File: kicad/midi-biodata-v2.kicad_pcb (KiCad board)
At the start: 2 copper layers, 63.5 x 45.7 mm, 37 parts, among them J1 DIN-5_180degree, J2 Audio-Jack-2, J3 Conn_01x02, J4 Conn_01x02, SW1 SW_Push, U1 ATMEGA328P-AU, U2 POT_SWITCH, U3 LMC555xM, Y1 Crystal_GND2

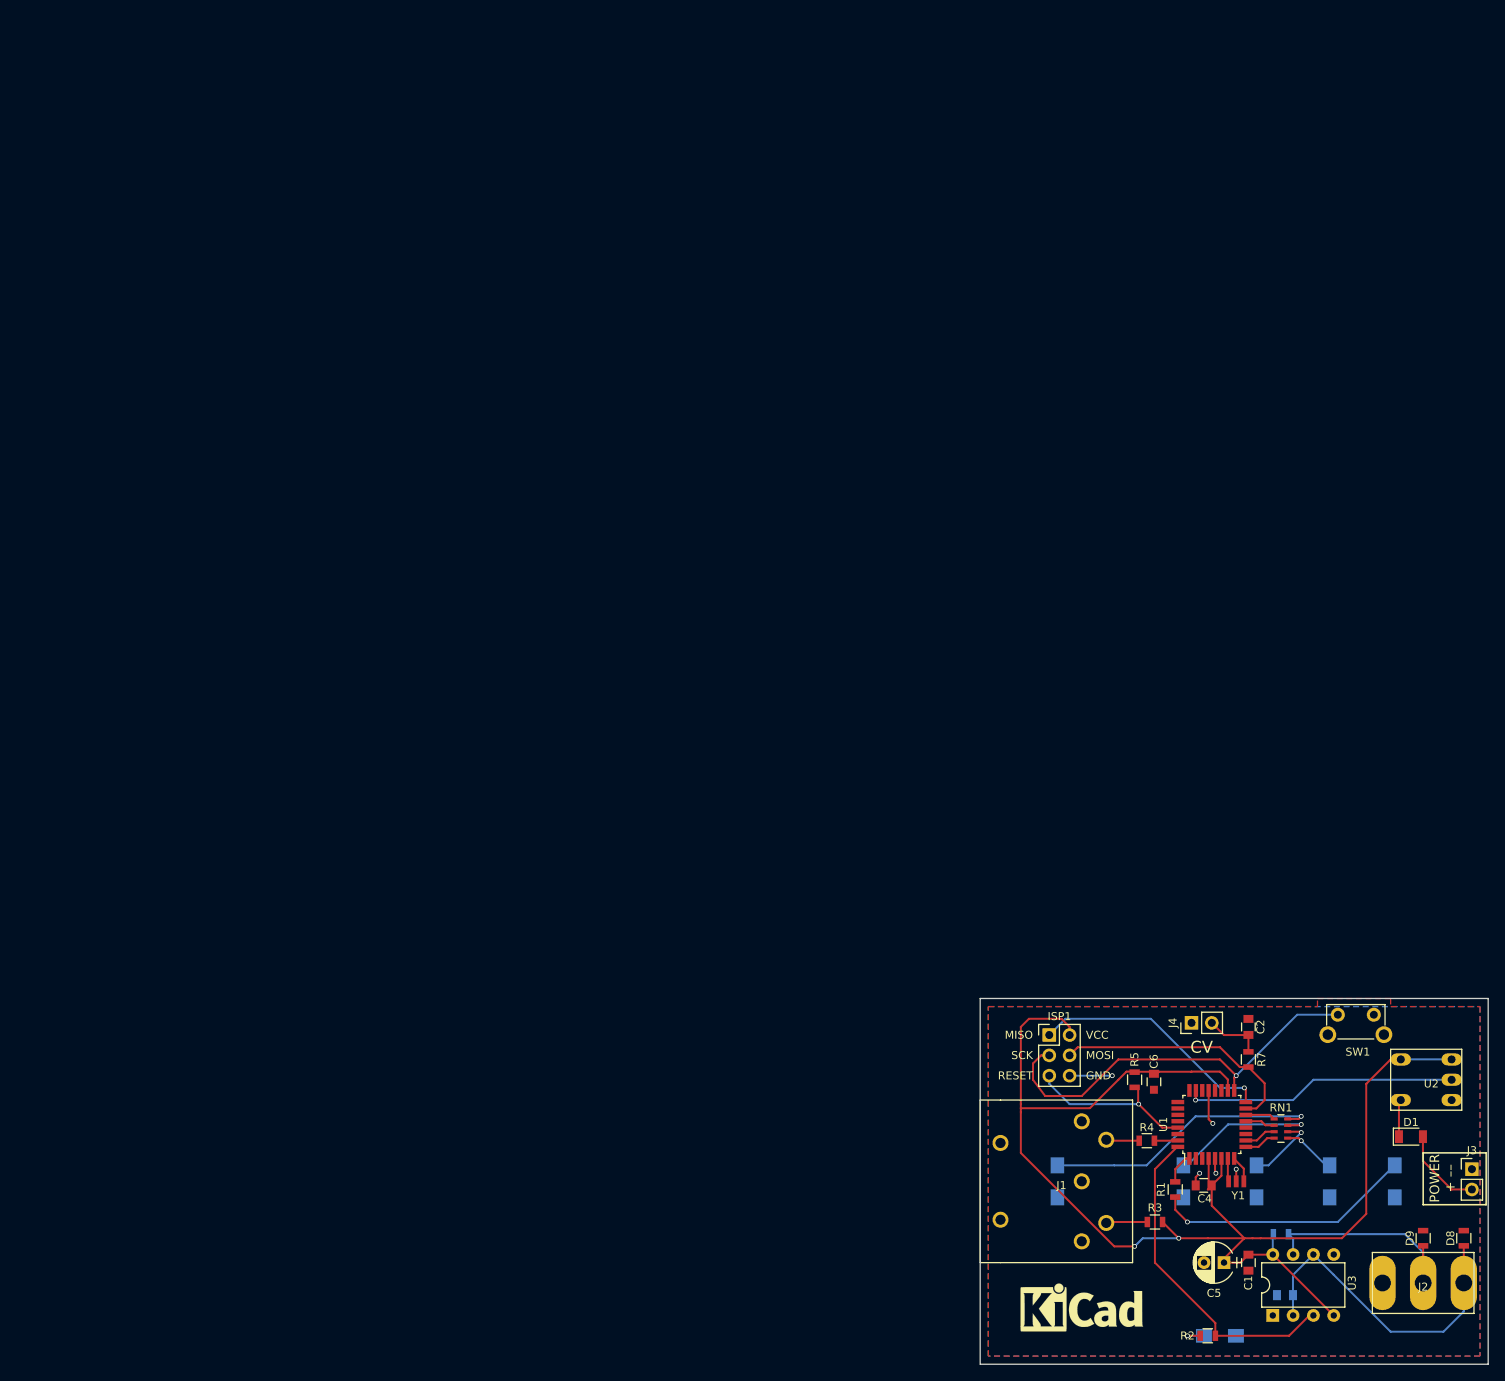
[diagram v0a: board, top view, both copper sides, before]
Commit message: upload v2.1
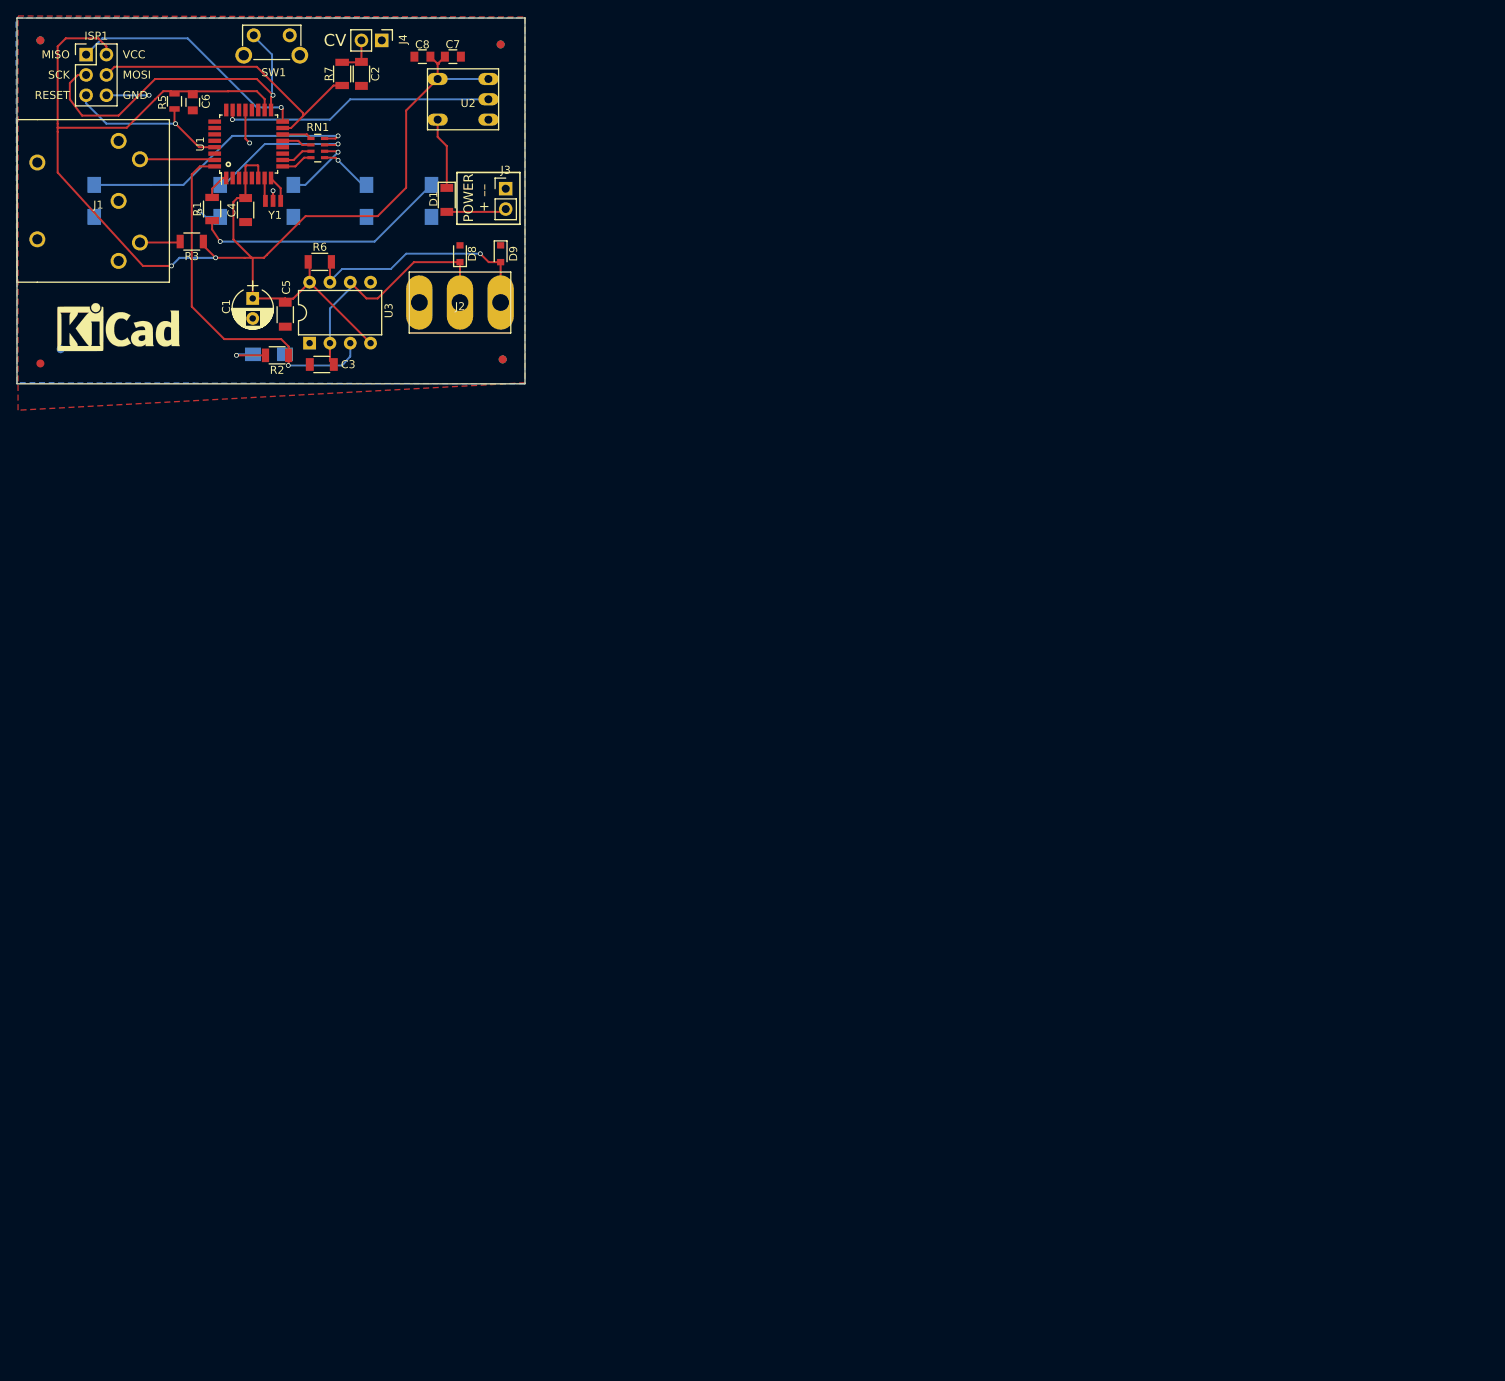
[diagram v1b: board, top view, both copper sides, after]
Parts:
- removed R4: 0R, Resistors_SMD:R_0805
- added ?: Fiducial_1mm_Dia_2.54mm_Outer_CopperBottom, Fiducials:Fiducial_1mm_Dia_2.54mm_Outer_CopperBottom, F.Cu at (5.46, -4.45)
- added ?: Fiducial_1mm_Dia_2.54mm_Outer_CopperBottom, Fiducials:Fiducial_1mm_Dia_2.54mm_Outer_CopperBottom, F.Cu at (2.92, -43.1)
- added ?: Fiducial_1mm_Dia_2.54mm_Outer_CopperBottom, Fiducials:Fiducial_1mm_Dia_2.54mm_Outer_CopperBottom, F.Cu at (60.5, -42.5)
- added ?: Fiducial_1mm_Dia_2.54mm_Outer_CopperBottom, Fiducials:Fiducial_1mm_Dia_2.54mm_Outer_CopperBottom, F.Cu at (60.7, -3.17)
- added ?: Fiducial_1mm_Dia_2.54mm_Outer_CopperTop, Fiducials:Fiducial_1mm_Dia_2.54mm_Outer_CopperTop, F.Cu at (2.92, -43.1)
- added ?: Fiducial_1mm_Dia_2.54mm_Outer_CopperTop, Fiducials:Fiducial_1mm_Dia_2.54mm_Outer_CopperTop, F.Cu at (2.92, -2.67)
- added ?: Fiducial_1mm_Dia_2.54mm_Outer_CopperTop, Fiducials:Fiducial_1mm_Dia_2.54mm_Outer_CopperTop, F.Cu at (60.7, -3.17)
- added ?: Fiducial_1mm_Dia_2.54mm_Outer_CopperTop, Fiducials:Fiducial_1mm_Dia_2.54mm_Outer_CopperTop, F.Cu at (60.5, -42.5)
- added C7: 100nF, Capacitors_SMD:C_0805, F.Cu at (54.5, -41.0)
- added C8: 1uF, Capacitors_SMD:C_0805, F.Cu at (50.7, -41.0)
- C1, C2, C4: footprint Capacitors_SMD:C_0805 -> Capacitors_SMD:C_1206
- C3: footprint Capacitors_SMD:C_0805 -> Capacitors_SMD:C_1206; moved to F.Cu
- D8, D9: footprint Resistors_SMD:R_0805 -> Diodes_SMD:D_0805
- R1, R2, R3, R7: footprint Resistors_SMD:R_0805 -> Resistors_SMD:R_1206
- R6: footprint Resistors_SMD:R_0805 -> Resistors_SMD:R_1206; moved to F.Cu
- moved SW1 182.6 mm to (29.6, -43.7)
- moved D8 175.8 mm to (55.4, -16.4)
- moved J3 172.1 mm to (61.1, -24.5)
- moved D2 171.8 mm to (9.65, -23.0)
- moved D4 171.8 mm to (34.5, -23.0)
- moved D5 171.8 mm to (43.7, -23.0)
- moved ISP1 171.8 mm to (8.64, -41.3)
- moved J1 171.8 mm to (10.2, -23.0)
- moved R3 171.8 mm to (21.8, -17.9)
- moved REF** 171.8 mm to (13.7, -8.26)
- moved Y1 171.8 mm to (32.0, -23.0)
- moved D3 171.8 mm to (25.4, -23.0)
- moved D6 171.8 mm to (51.8, -23.0)
- moved G*** 171.8 mm to (23.9, -11.8)
- moved J2 171.8 mm to (55.4, -10.3)
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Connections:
- J1 pad 1: (no net) -> Net-(J1-Pad1)
- J1 pad 3: (no net) -> Net-(J1-Pad3)
- J2 pad 1: Net-(C3-Pad2) -> Net-(D9-Pad2)
- J2 pad 2: Net-(D9-Pad2) -> Net-(C3-Pad2)
- U1 pad 11: (no net) -> Net-(U1-Pad11)
- U1 pad 12: (no net) -> Net-(U1-Pad12)
- U1 pad 19: (no net) -> Net-(U1-Pad19)
- U1 pad 2: (no net) -> Net-(U1-Pad2)
- U1 pad 20: (no net) -> Net-(U1-Pad20)
- U1 pad 22: (no net) -> Net-(U1-Pad22)
- U1 pad 24: (no net) -> Net-(U1-Pad24)
- U1 pad 25: (no net) -> Net-(U1-Pad25)
- U1 pad 26: (no net) -> Net-(U1-Pad26)
- U1 pad 27: (no net) -> Net-(U1-Pad27)
- U1 pad 28: (no net) -> Net-(U1-Pad28)
- U1 pad 30: (no net) -> Net-(U1-Pad30)
- U1 pad 31: Net-(R4-Pad2) -> Net-(J1-Pad5)
- U3 pad 5: (no net) -> Net-(U3-Pad5)
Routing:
- net Net-(C3-Pad2): track 43.3 -> 33.6 mm
- net SCK: track 52.1 -> 44.8 mm
- net Net-(J1-Pad5): track 3.41 -> 9.42 mm
- net MOSI: track 31.6 -> 37.4 mm
- net 555: track 41.3 -> 46.7 mm, vias 0 -> 1
- net +5V: track 4.67 -> 9.33 mm
- net Net-(D9-Pad2): track 29.0 -> 33.6 mm, vias 0 -> 1
- net VCC: track 175.1 -> 179.3 mm
- net Net-(R4-Pad2): track 2.94 -> 0.00 mm
- net Net-(D1-Pad2): track 10.6 -> 7.89 mm
- net Net-(C2-Pad1): track 7.32 -> 5.12 mm
- net Net-(D7-Pad2): track 3.65 -> 5.75 mm
- net GND: track 14.8 -> 13.8 mm, vias 5 -> 4
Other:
- board text added: "13-37.org electronics MIDI Biodata Sonification Device (2.1.1)"
- board text added: "B"
- board text added: "G"
- board text added: "R"
- board text added: "W"
- board text added: "Y"
- board text removed: "13-37.org electronics MIDI Biodata Sonification Device (2.0)"
